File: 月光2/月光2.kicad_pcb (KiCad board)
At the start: 2 copper layers, 40 x 60.5 mm, 73 parts, among them J1 Conn_01x12, J2 Conn_01x12, J3 Conn_01x05, J4 Conn_01x03, J6 Conn_01x02, Q1 Q_Photo_NPN, Q2 Q_Photo_NPN, Q3 Q_Photo_NPN, Q4 Q_Photo_NPN, Q5 IRLML6344TRPBFTR, SW1 SW_Push_Dual_x2, U1 DRV8835, U2 STM32F413CH6, U4 LP5907_DBV, U5 ICM20648, Y1 Crystal_GND23

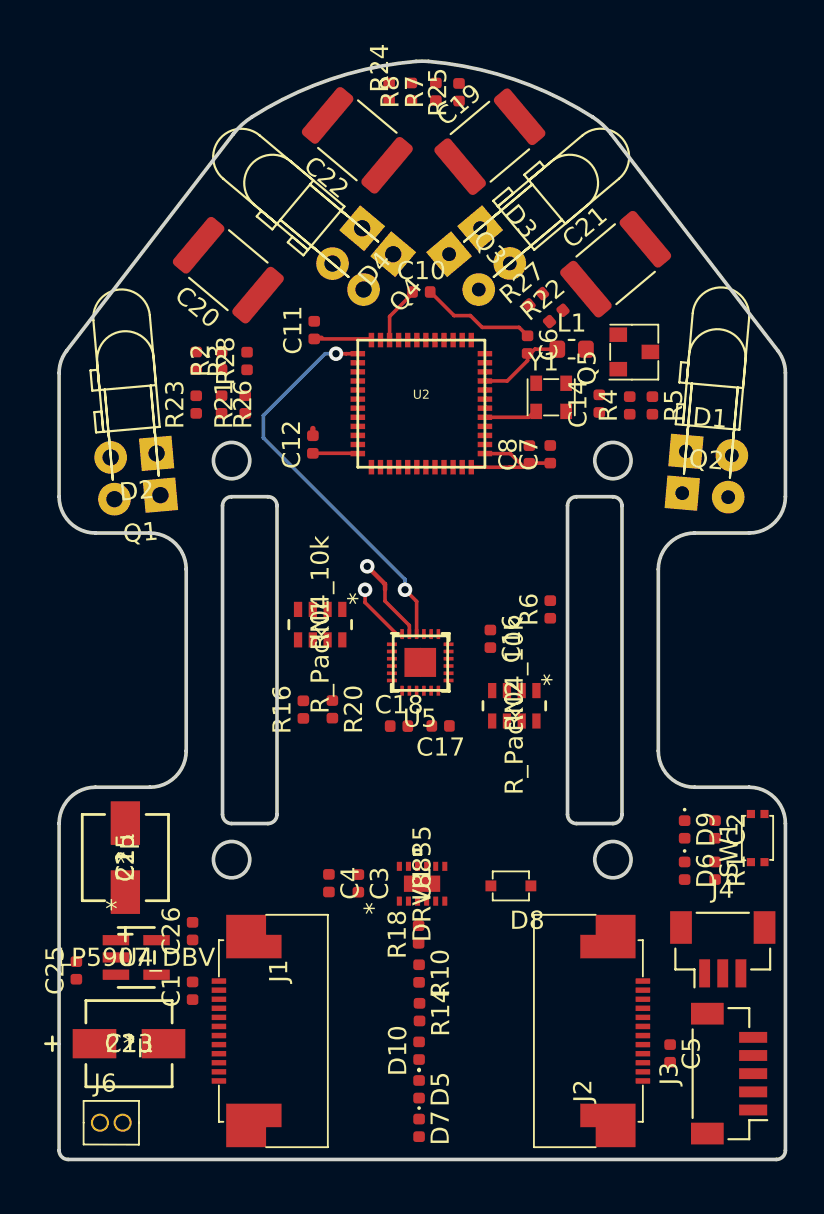
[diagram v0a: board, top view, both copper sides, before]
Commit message: ##
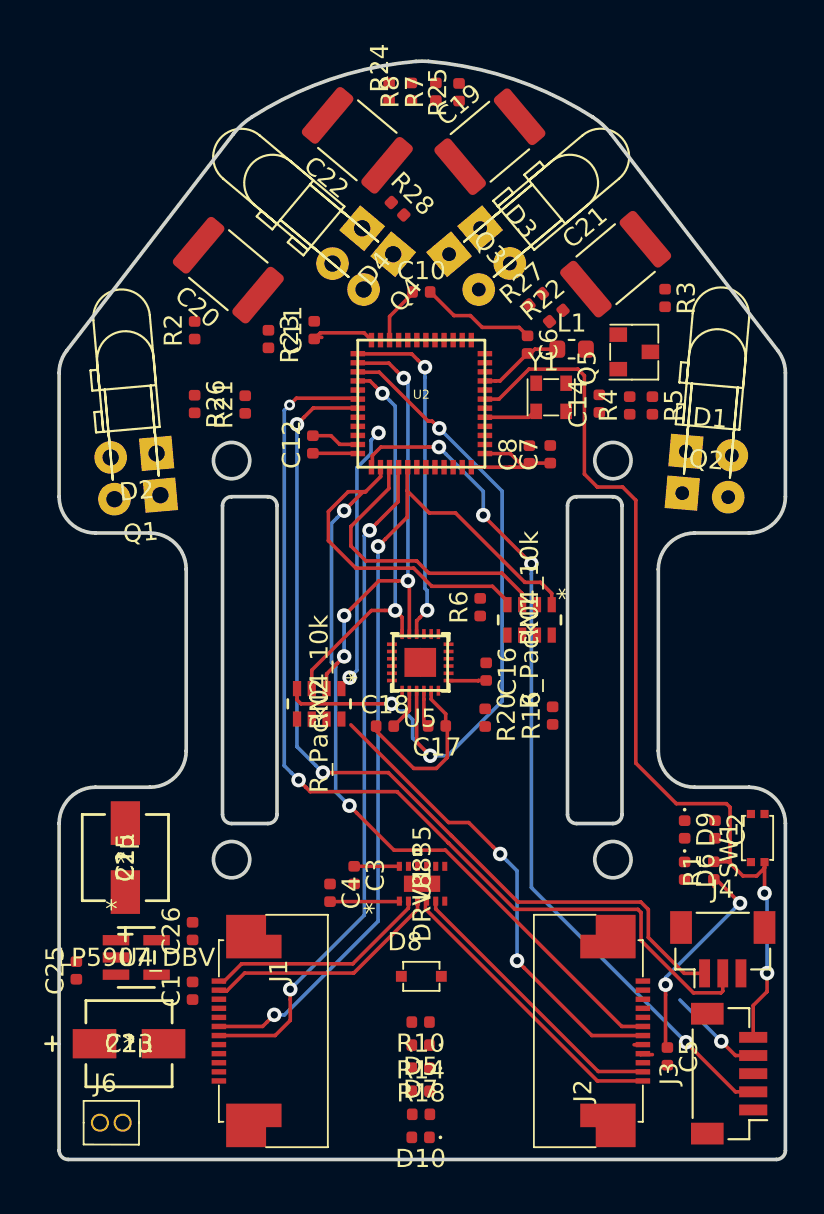
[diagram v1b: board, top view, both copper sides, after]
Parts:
- moved R3 26.1 mm to (163.3, 100.3)
- moved R16 13.7 mm to (157.1, 123.3)
- moved R28 11.8 mm to (148.6, 95.4), turned to 315 degrees
- moved RN1 11.5 mm to (155.9, 118.1)
- moved RN2 10.7 mm to (144.3, 122.7)
- moved R18 9.90 mm to (149.9, 145.3), turned to 0 degrees
- moved R20 8.43 mm to (153.4, 123.4)
- moved D8 7.01 mm to (149.9, 137.7), turned to 180 degrees
- moved R23 5.37 mm to (141.5, 102.6), turned to 270 degrees
- moved D10 4.77 mm to (149.9, 146.6), turned to 180 degrees
- moved R14 4.36 mm to (149.9, 144.0), turned to 0 degrees
- moved R6 3.86 mm to (153.1, 117.4)
- moved D7 3.29 mm to (149.9, 142.7), turned to 180 degrees
- moved R10 2.67 mm to (149.9, 140.2), turned to 180 degrees
- moved D5 2.43 mm to (149.9, 141.5), turned to 180 degrees
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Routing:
- net encL_2: track 0.00 -> 56.8 mm, vias 0 -> 2
- net UART_TX: track 0.00 -> 55.0 mm, vias 0 -> 2
- net NRST: track 0.00 -> 52.8 mm, vias 0 -> 2
- net UART_RX: track 0.00 -> 49.9 mm, vias 0 -> 2
- net encR_1: track 0.00 -> 47.8 mm, vias 0 -> 2
- net STLINK_TCK: track 0.00 -> 47.6 mm, vias 0 -> 4
- net encL_1: track 0.00 -> 42.2 mm, vias 0 -> 2
- net MISO_IMU: track 0.00 -> 41.1 mm, vias 0 -> 3
- net encR_2: track 0.00 -> 37.0 mm, vias 0 -> 2
- net SCK_IMU: track 4.69 -> 25.7 mm, vias 1 -> 4
- net MOSI_IMU: track 3.46 -> 22.3 mm, vias 1 -> 2
- net +3V3: track 9.75 -> 26.7 mm, vias 0 -> 2
- net MORTOR_2+: track 0.00 -> 16.3 mm
- net MORTOR_2-: track 0.00 -> 15.7 mm
- net MORTOR_1-: track 0.00 -> 13.2 mm
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
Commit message: finish
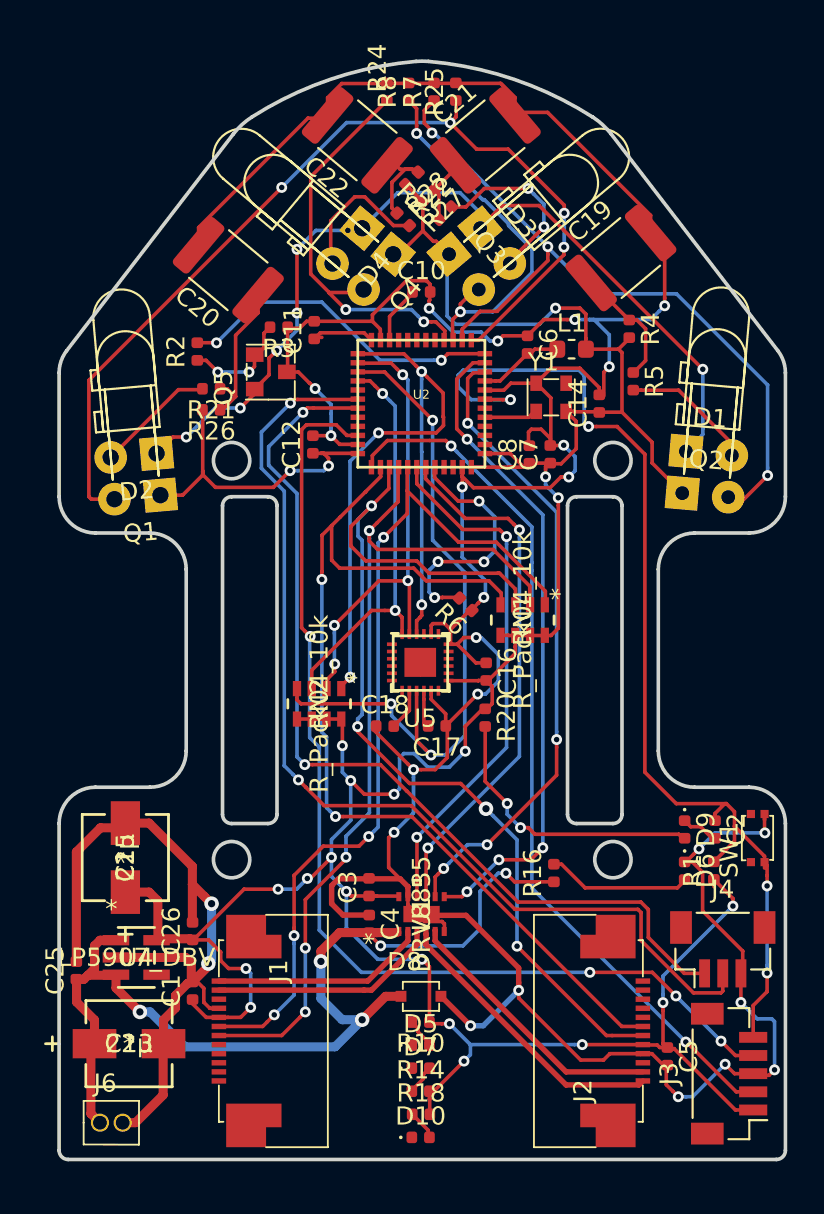
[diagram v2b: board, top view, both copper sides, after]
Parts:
- moved R3 21.3 mm to (142.1, 101.9), turned to 180 degrees
- moved Q5 20.1 mm to (143.0, 104.4)
- moved R23 9.93 mm to (148.9, 96.0), turned to 315 degrees
- moved C21 9.90 mm to (153.4, 91.7)
- moved C19 9.65 mm to (160.9, 98.1)
- moved R16 8.67 mm to (157.2, 132.0)
- moved R22 8.34 mm to (151.2, 95.7), turned to 45 degrees
- moved R27 8.21 mm to (150.3, 94.7), turned to 225 degrees
- moved R4 4.22 mm to (161.3, 102.0), turned to 270 degrees
- moved C4 2.75 mm to (147.0, 134.8)
- moved R21 2.06 mm to (138.3, 105.3), turned to 180 degrees
- moved R28 1.85 mm to (149.4, 93.7), turned to 225 degrees
- moved R5 1.70 mm to (161.6, 104.9)
- moved U1 1.67 mm to (149.9, 134.3)
- moved R2 1.18 mm to (137.6, 103.3)
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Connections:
- U2 pad 42: MotorR_Foward -> MotorR_Reverce
- U2 pad 43: MotorR_Reverce -> MotorR_Foward
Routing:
- net GND: track 18.3 -> 247.9 mm, vias 0 -> 25
- net +3V3: track 26.7 -> 183.2 mm, vias 2 -> 21
- net sens_RR: track 0.00 -> 52.9 mm, vias 0 -> 4
- net STLINK_TMS: track 5.30 -> 58.2 mm, vias 1 -> 4
- net +BATT: track 3.88 -> 55.6 mm, vias 0 -> 5
- net Net-(D1-Pad1): track 0.00 -> 48.4 mm, vias 0 -> 7
- net sens_R: track 0.00 -> 41.1 mm, vias 0 -> 3
- net MotorL_Foward: track 0.00 -> 36.2 mm, vias 0 -> 4
- net MotorL_Reverce: track 0.00 -> 35.1 mm, vias 0 -> 4
- net MotorR_Foward: track 0.00 -> 29.3 mm, vias 0 -> 2
- net MotorR_Reverce: track 0.00 -> 28.8 mm, vias 0 -> 2
- net sens_LL: track 0.00 -> 21.7 mm, vias 0 -> 2
- net sens_L: track 0.00 -> 20.6 mm, vias 0 -> 2
- net RLED_PWM: track 0.00 -> 18.2 mm, vias 0 -> 2
- net Net-(D9-Pad2): track 0.00 -> 15.6 mm, vias 0 -> 2
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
